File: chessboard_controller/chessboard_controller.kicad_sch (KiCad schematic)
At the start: 18 parts, among them J1 Conn_01x04, J2 Conn_01x06, J3 Conn_01x08, J4 Conn_01x08, J5 Conn_01x10, J6 Conn_02x32_Counter_Clockwise, U1 HV4067, U2 HV4067, U3 HV4067, U4 HV4067

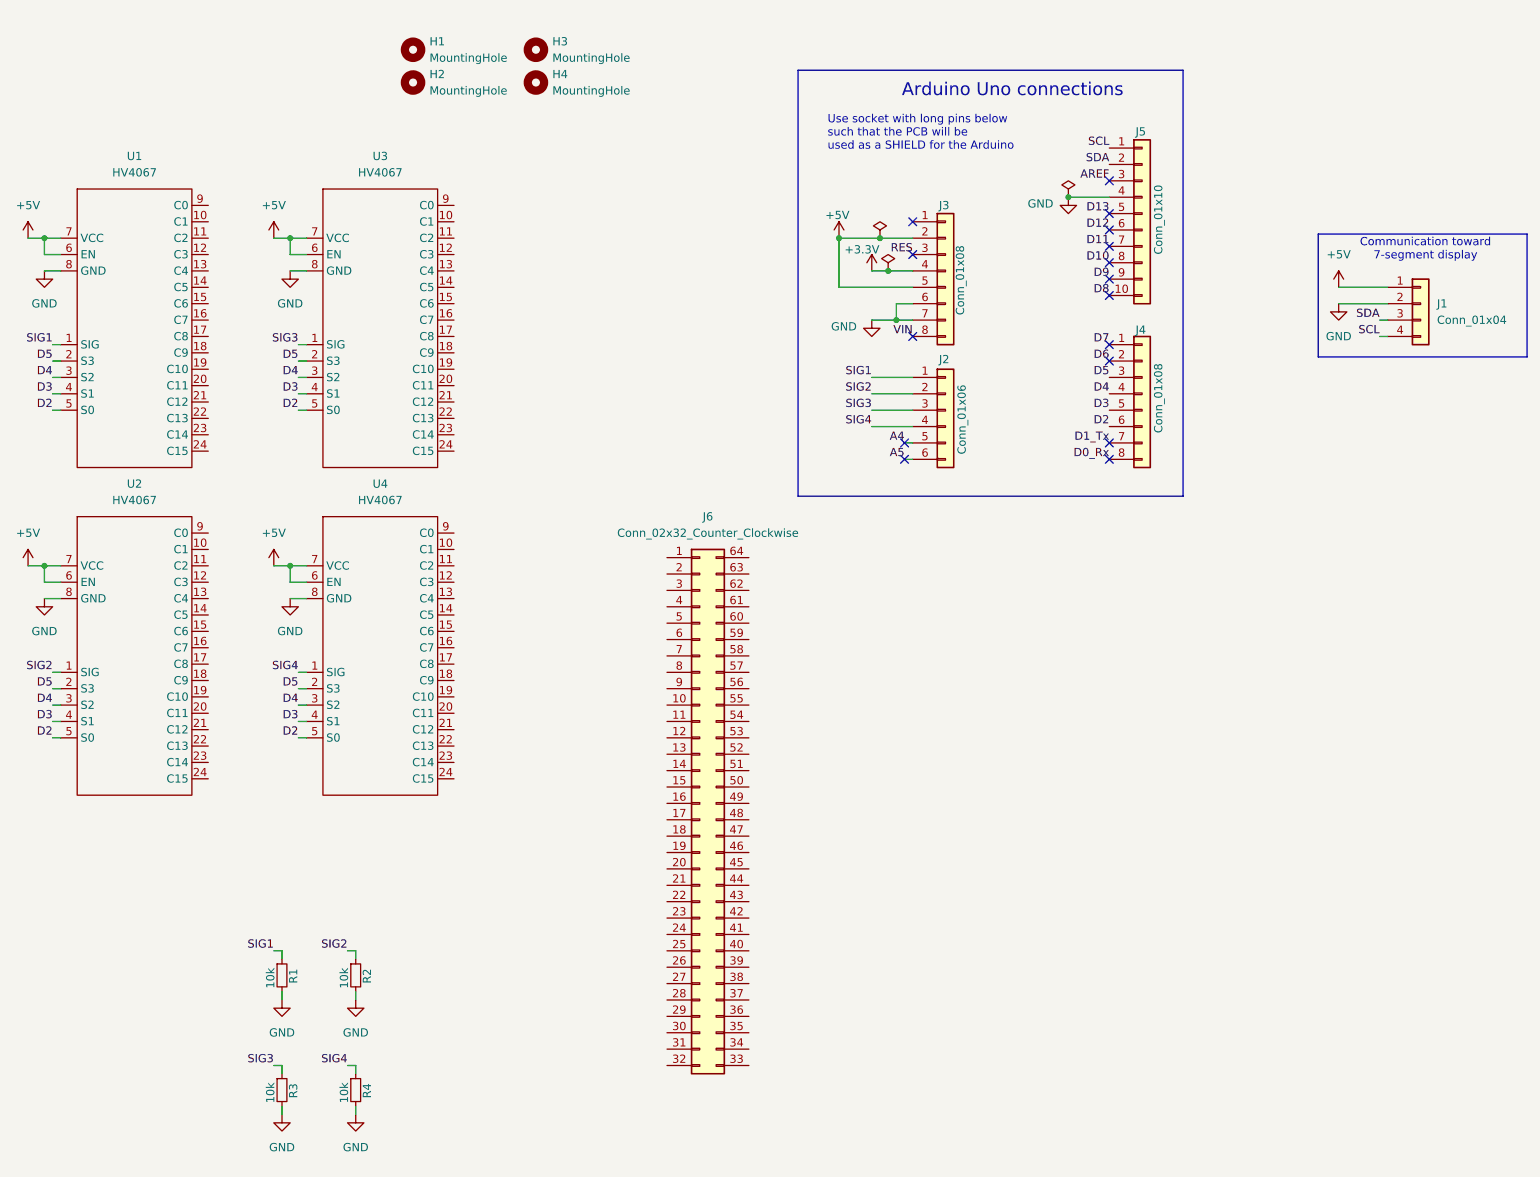
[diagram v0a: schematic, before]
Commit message: First version of layout
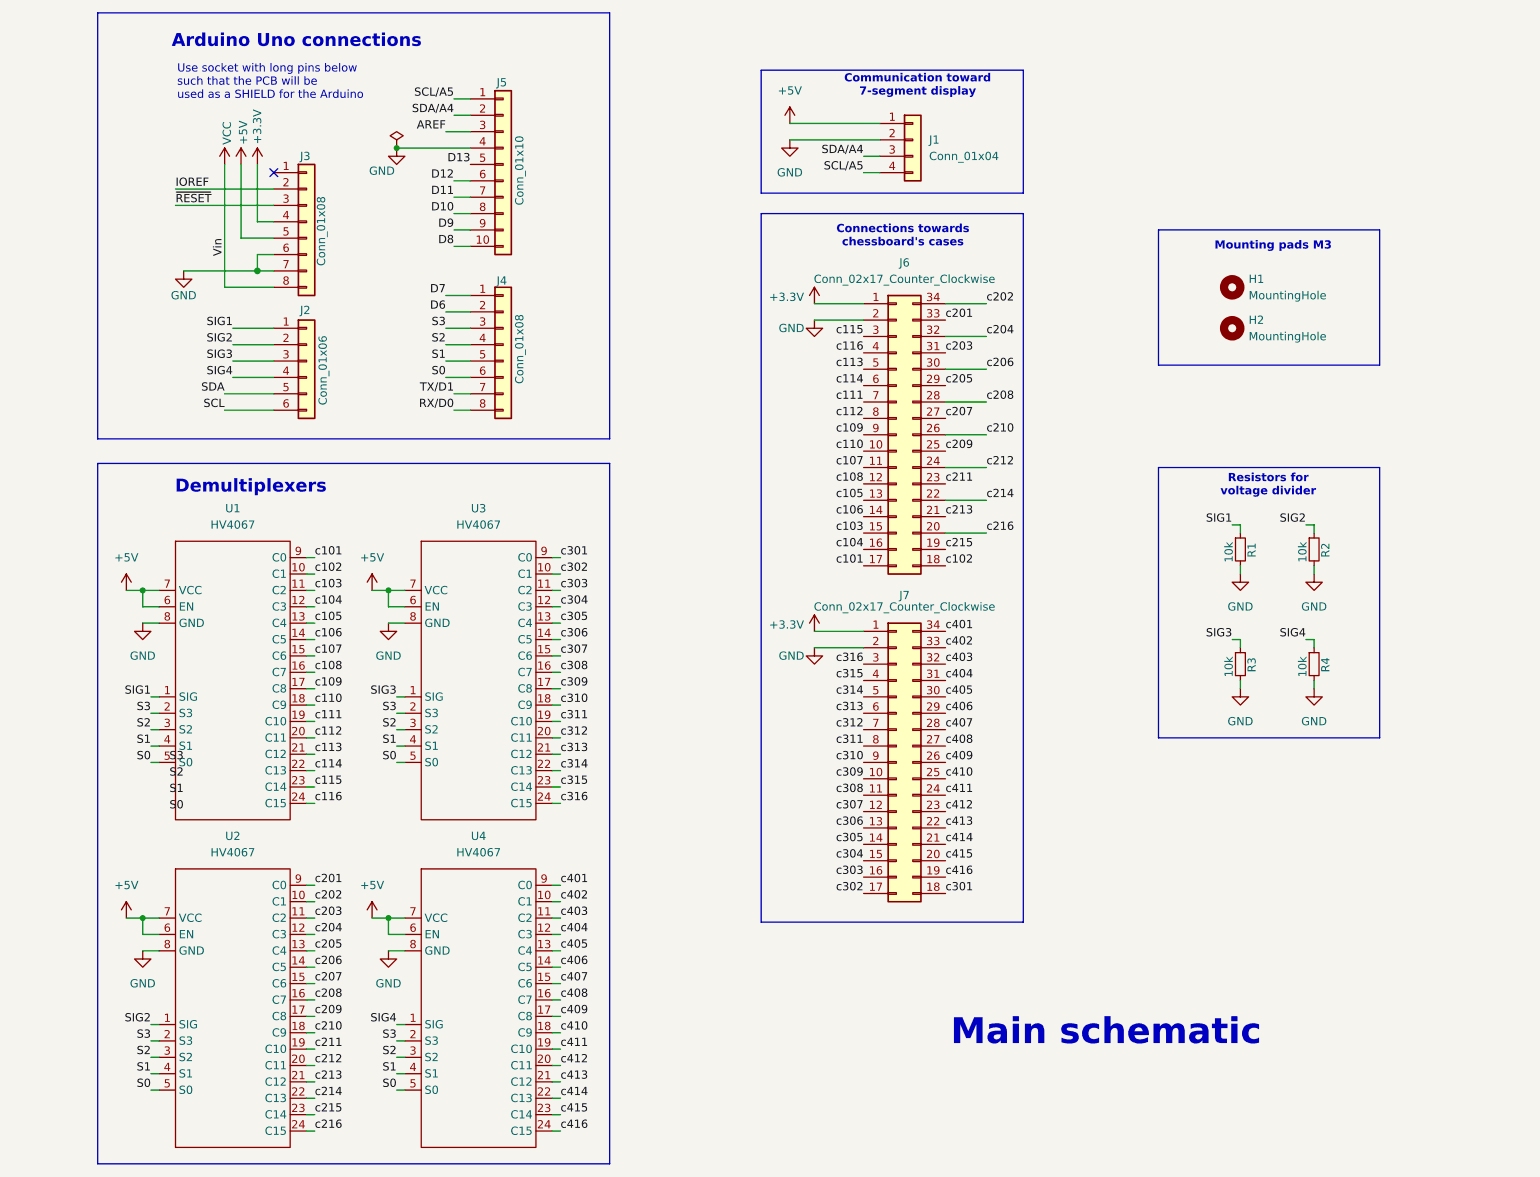
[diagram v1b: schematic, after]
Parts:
- removed H3, H4: MountingHole, MountingHole:MountingHole_3.2mm_M3, symbol Mechanical:MountingHole
- removed J6: Conn_02x32_Counter_Clockwise, symbol Connector_Generic:Conn_02x32_Counter_Clockwise
- added J6, J7: Conn_02x17_Counter_Clockwise, Connector_IDC:IDC-Header_2x17_P2.54mm_Horizontal, symbol Connector_Generic:Conn_02x17_Counter_Clockwise
- H1, H2: footprint MountingHole:MountingHole_3.2mm_M3 -> MountingHole:MountingHole_3.2mm_M3_ISO7380
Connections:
- net A4 is gone; now on net SDA: J2.5 (Pin_5)
- net A5 is gone; now on net SCL: J2.6 (Pin_6)
- net +3.3V: now also J6.1 (Pin_1), J7.1 (Pin_1)
- net +5V: no longer J3.2 (Pin_2)
- net GND: now also J6.2 (Pin_2), J7.2 (Pin_2)
- net SCL: no longer J1.4 (Pin_4), J5.1 (Pin_1)
- net SDA: no longer J1.3 (Pin_3), J5.2 (Pin_2)
- net c302: now reaches U3.10 (C1)
- net c302: now also J7.17 (Pin_17)
- net c303: now reaches U3.11 (C2)
- net c303: now also J7.16 (Pin_16)
- net c304: now reaches U3.12 (C3)
- net c304: now also J7.15 (Pin_15)
- net c305: now reaches U3.13 (C4)
- net c305: now also J7.14 (Pin_14)
- net c306: now reaches U3.14 (C5)
- net c306: now also J7.13 (Pin_13)
- net c307: now reaches U3.15 (C6)
- net c307: now also J7.12 (Pin_12)
- net c308: now reaches U3.16 (C7)
- net c308: now also J7.11 (Pin_11)
- net c309: now reaches U3.17 (C8)
- net c309: now also J7.10 (Pin_10)
- net c310: now reaches U3.18 (C9)
- net c310: now also J7.9 (Pin_9)
- net c311: now reaches U3.19 (C10)
- net c311: now also J7.8 (Pin_8)
- net c312: now reaches U3.20 (C11)
- net c312: now also J7.7 (Pin_7)
- net c313: now reaches U3.21 (C12)
- net c313: now also J7.6 (Pin_6)
- net c314: now reaches U3.22 (C13)
- net c314: now also J7.5 (Pin_5)
- net c315: now reaches U3.23 (C14)
- net c315: now also J7.4 (Pin_4)
- net c316: now reaches U3.24 (C15)
- net c316: now also J7.3 (Pin_3)
- net c301: now reaches U3.9 (C0)
- net c301: now also J7.18 (Pin_18)
- net c202: now reaches U2.10 (C1)
- net c202: now also J6.34 (Pin_34)
- net c203: now reaches U2.11 (C2)
- net c203: now also J6.31 (Pin_31)
- net c204: now reaches U2.12 (C3)
- net c204: now also J6.32 (Pin_32)
- net c205: now reaches U2.13 (C4)
- net c205: now also J6.29 (Pin_29)
- net c206: now reaches U2.14 (C5)
- net c206: now also J6.30 (Pin_30)
- net c207: now reaches U2.15 (C6)
- net c207: now also J6.27 (Pin_27)
- net c208: now reaches U2.16 (C7)
- net c208: now also J6.28 (Pin_28)
- net c209: now reaches U2.17 (C8)
- net c209: now also J6.25 (Pin_25)
- net c210: now reaches U2.18 (C9)
- net c210: now also J6.26 (Pin_26)
- net c211: now reaches U2.19 (C10)
- net c211: now also J6.23 (Pin_23)
- net c212: now reaches U2.20 (C11)
- net c212: now also J6.24 (Pin_24)
- net c213: now reaches U2.21 (C12)
- net c213: now also J6.21 (Pin_21)
- net c214: now reaches U2.22 (C13)
- net c214: now also J6.22 (Pin_22)
- net c215: now reaches U2.23 (C14)
- net c215: now also J6.19 (Pin_19)
- net c216: now reaches U2.24 (C15)
- net c216: now also J6.20 (Pin_20)
- net c201: now reaches U2.9 (C0)
- net c201: now also J6.33 (Pin_33)
- net c402: now reaches U4.10 (C1)
- net c402: now also J7.33 (Pin_33)
- net c403: now reaches U4.11 (C2)
- net c403: now also J7.32 (Pin_32)
- net c404: now reaches U4.12 (C3)
- net c404: now also J7.31 (Pin_31)
- net c405: now reaches U4.13 (C4)
- net c405: now also J7.30 (Pin_30)
- net c406: now reaches U4.14 (C5)
- net c406: now also J7.29 (Pin_29)
- net c407: now reaches U4.15 (C6)
- net c407: now also J7.28 (Pin_28)
- net c408: now reaches U4.16 (C7)
- net c408: now also J7.27 (Pin_27)
- net c409: now reaches U4.17 (C8)
- net c409: now also J7.26 (Pin_26)
- net c410: now reaches U4.18 (C9)
- net c410: now also J7.25 (Pin_25)
- net c411: now reaches U4.19 (C10)
- net c411: now also J7.24 (Pin_24)
- net c412: now reaches U4.20 (C11)
- net c412: now also J7.23 (Pin_23)
- net c413: now reaches U4.21 (C12)
- net c413: now also J7.22 (Pin_22)
- net c414: now reaches U4.22 (C13)
- net c414: now also J7.21 (Pin_21)
- net c415: now reaches U4.23 (C14)
- net c415: now also J7.20 (Pin_20)
- net c416: now reaches U4.24 (C15)
- net c416: now also J7.19 (Pin_19)
- net c401: now reaches U4.9 (C0)
- net c401: now also J7.34 (Pin_34)
- net c102: now reaches U1.10 (C1)
- net c102: now also J6.18 (Pin_18)
- net c103: now reaches U1.11 (C2)
- net c103: now also J6.15 (Pin_15)
- net c104: now reaches U1.12 (C3)
- net c104: now also J6.16 (Pin_16)
- net c105: now reaches U1.13 (C4)
- net c105: now also J6.13 (Pin_13)
- net c106: now reaches U1.14 (C5)
- net c106: now also J6.14 (Pin_14)
- net c107: now reaches U1.15 (C6)
- net c107: now also J6.11 (Pin_11)
- net c108: now reaches U1.16 (C7)
- net c108: now also J6.12 (Pin_12)
- net c109: now reaches U1.17 (C8)
- net c109: now also J6.9 (Pin_9)
- net c110: now reaches U1.18 (C9)
- net c110: now also J6.10 (Pin_10)
- net c111: now reaches U1.19 (C10)
- net c111: now also J6.7 (Pin_7)
- net c112: now reaches U1.20 (C11)
- net c112: now also J6.8 (Pin_8)
- net c113: now reaches U1.21 (C12)
- net c113: now also J6.5 (Pin_5)
- net c114: now reaches U1.22 (C13)
- net c114: now also J6.6 (Pin_6)
- net c115: now reaches U1.23 (C14)
- net c115: now also J6.3 (Pin_3)
- net c116: now reaches U1.24 (C15)
- net c116: now also J6.4 (Pin_4)
- net c101: now reaches U1.9 (C0)
- net c101: now also J6.17 (Pin_17)
- net D0_Rx renamed RX/D0
- net D1_Tx renamed TX/D1
- net D2 renamed S0
- net D3 renamed S1
- net D4 renamed S2
- net D5 renamed S3
- net RES renamed ~{RESET}
- net VIN renamed VCC
- new net IOREF: J3.2 (Pin_2)
- new net SCL/A5: J1.4 (Pin_4), J5.1 (Pin_1)
- new net SDA/A4: J1.3 (Pin_3), J5.2 (Pin_2)
- no-connect marks 16 -> 1
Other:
- note added: "Connections towards chessboard's cases"
- note added: "Demultiplexers"
- note added: "Main schematic"
- note added: "Mounting pads M3"
- note added: "Resistors for voltage divider"
- title: (none) -> Arduino Shield Chessboard Controller
- moved on the sheet: J1, J2, J3, J4, J5, R1, R2, R3, R4, U1, U2, U3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
